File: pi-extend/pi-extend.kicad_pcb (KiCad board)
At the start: 2 copper layers, 53.3 x 67.1 mm, 5 parts, among them J1 Conn_02x20_Odd_Even, J2 Conn_01x20_Male, J3 Conn_01x20_Male, J4 Conn_01x02_Male, J5 Conn_01x02_Male

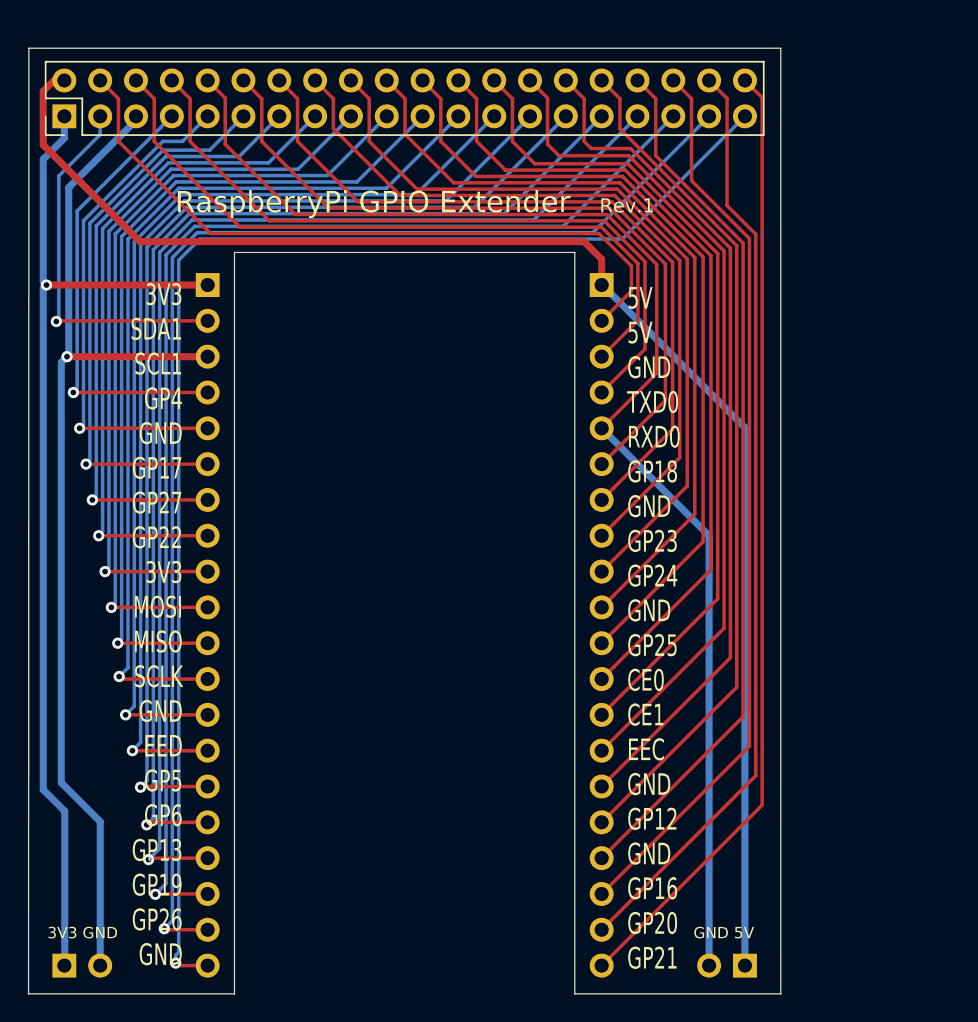
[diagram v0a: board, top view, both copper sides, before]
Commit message: pi extender 레이아웃 축소
Signed-off-by: Ju, Gyeong-min <jcmh74@gmail.com>
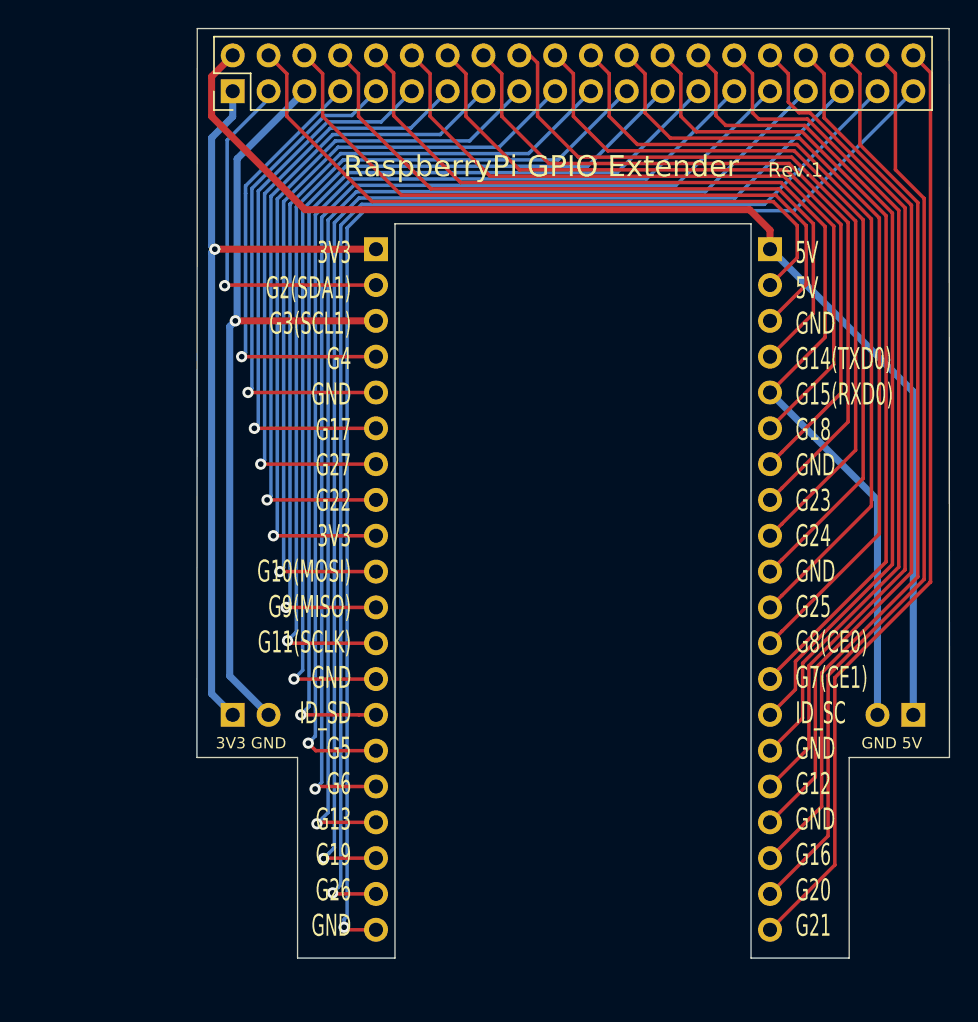
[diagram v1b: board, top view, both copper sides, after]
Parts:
- moved J4 21.4 mm to (138.7, 111.8)
- moved J5 21.4 mm to (186.9, 111.8)
- moved J2 12.2 mm to (148.8, 78.8)
- moved J3 12.2 mm to (176.8, 78.8)
- moved J1 12.1 mm to (138.7, 67.6)
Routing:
- net Net-(J1-Pad2): track 102.9 -> 86.5 mm
- net Net-(J1-Pad1): track 73.1 -> 57.1 mm
- net Net-(J1-Pad5): track 73.5 -> 57.5 mm
- net Net-(J1-Pad10): track 93.7 -> 78.0 mm
- net Net-(J1-Pad29): track 76.8 -> 76.0 mm
- net Net-(J1-Pad7): track 32.0 -> 31.2 mm
- net Net-(J1-Pad40): track 68.0 -> 67.2 mm
- net Net-(J1-Pad3): track 26.6 -> 25.8 mm
- net Net-(J1-Pad38): track 66.1 -> 65.4 mm
- net Net-(J1-Pad34): track 62.4 -> 61.6 mm
- net Net-(J1-Pad36): track 64.3 -> 63.5 mm
- net Net-(J1-Pad18): track 55.5 -> 56.1 mm
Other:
- board size 53.3 x 67.1 mm -> 53.4 x 65.9 mm
- board text added: "3V3 G2(SDA1) G3(SCL1) G4 GND G17 G27 G22 3V3 G10(MOSI) G9(MISO) G11(SCLK) GND ID_SD G5 G6 G13 G19 G26 GND"
- board text added: "5V 5V GND G14(TXD0) G15(RXD0) G18 GND G23 G24 GND G25 G8(CE0) G7(CE1) ID_SC GND G12 GND G16 G20 G21"
- board text removed: "3V3 SDA1 SCL1 GP4 GND GP17 GP27 GP22 3V3 MOSI MISO SCLK GND EED GP5 GP6 GP13 GP19 GP26 GND"
- board text removed: "5V 5V GND TXD0 RXD0 GP18 GND GP23 GP24 GND GP25 CE0 CE1 EEC GND GP12 GND GP16 GP20 GP21"
